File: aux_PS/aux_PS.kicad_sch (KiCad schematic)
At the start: 15 parts, among them J1 P78E03-1000, J2 Conn_02x03_Counter_Clockwise

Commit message: controller_final
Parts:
- AC_DC1, AC_DC2: footprint PSK-S6C-24:PSK-S6C-24 -> PSK-S6C-24:PSKS6C24
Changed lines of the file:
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@@
     (property "Reference" "AC_DC2" (id 0) (at 65.405 55.88 0))
     (property "Value" "PSK-S6C-24" (id 1) (at 65.405 58.42 0))
-    (property "Footprint" "PSK-S6C-24:PSK-S6C-24" (id 2) (at 68.58 71.12 0)
+    (property "Footprint" "PSK-S6C-24:PSKS6C24" (id 2) (at 68.58 71.12 0)
       (effects (font (size 1.27 1.27)) hide)
     )
@@
     (property "Reference" "AC_DC1" (id 0) (at 65.405 38.1 0))
     (property "Value" "PSK-S6C-24" (id 1) (at 65.405 40.64 0))
-    (property "Footprint" "PSK-S6C-24:PSK-S6C-24" (id 2) (at 68.58 53.34 0)
+    (property "Footprint" "PSK-S6C-24:PSKS6C24" (id 2) (at 68.58 53.34 0)
       (effects (font (size 1.27 1.27)) hide)
     )
@@
   (symbol_instances
     (path "/ab1d88f5-8232-454e-a102-ba9788c47905"
-      (reference "AC_DC1") (unit 1) (value "PSK-S6C-24") (footprint "PSK-S6C-24:PSK-S6C-24")
+      (reference "AC_DC1") (unit 1) (value "PSK-S6C-24") (footprint "PSK-S6C-24:PSKS6C24")
     )
     (path "/924609b2-ed56-4d39-928a-34e8ebf74acc"
-      (reference "AC_DC2") (unit 1) (value "PSK-S6C-24") (footprint "PSK-S6C-24:PSK-S6C-24")
+      (reference "AC_DC2") (unit 1) (value "PSK-S6C-24") (footprint "PSK-S6C-24:PSKS6C24")
     )
     (path "/c187c878-09da-4d9b-898f-142200e6ed75"

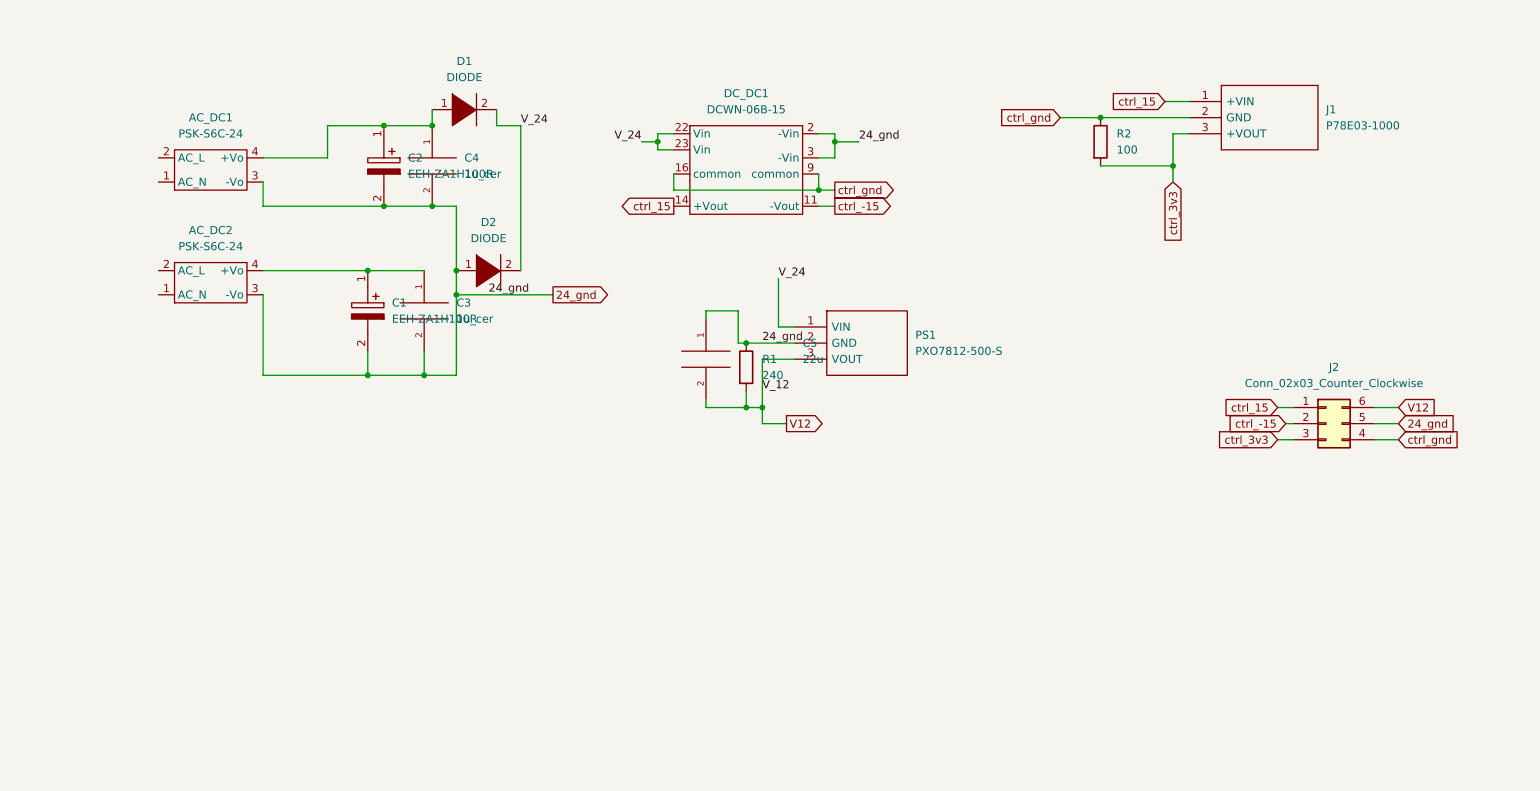
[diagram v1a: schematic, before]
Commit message: header design
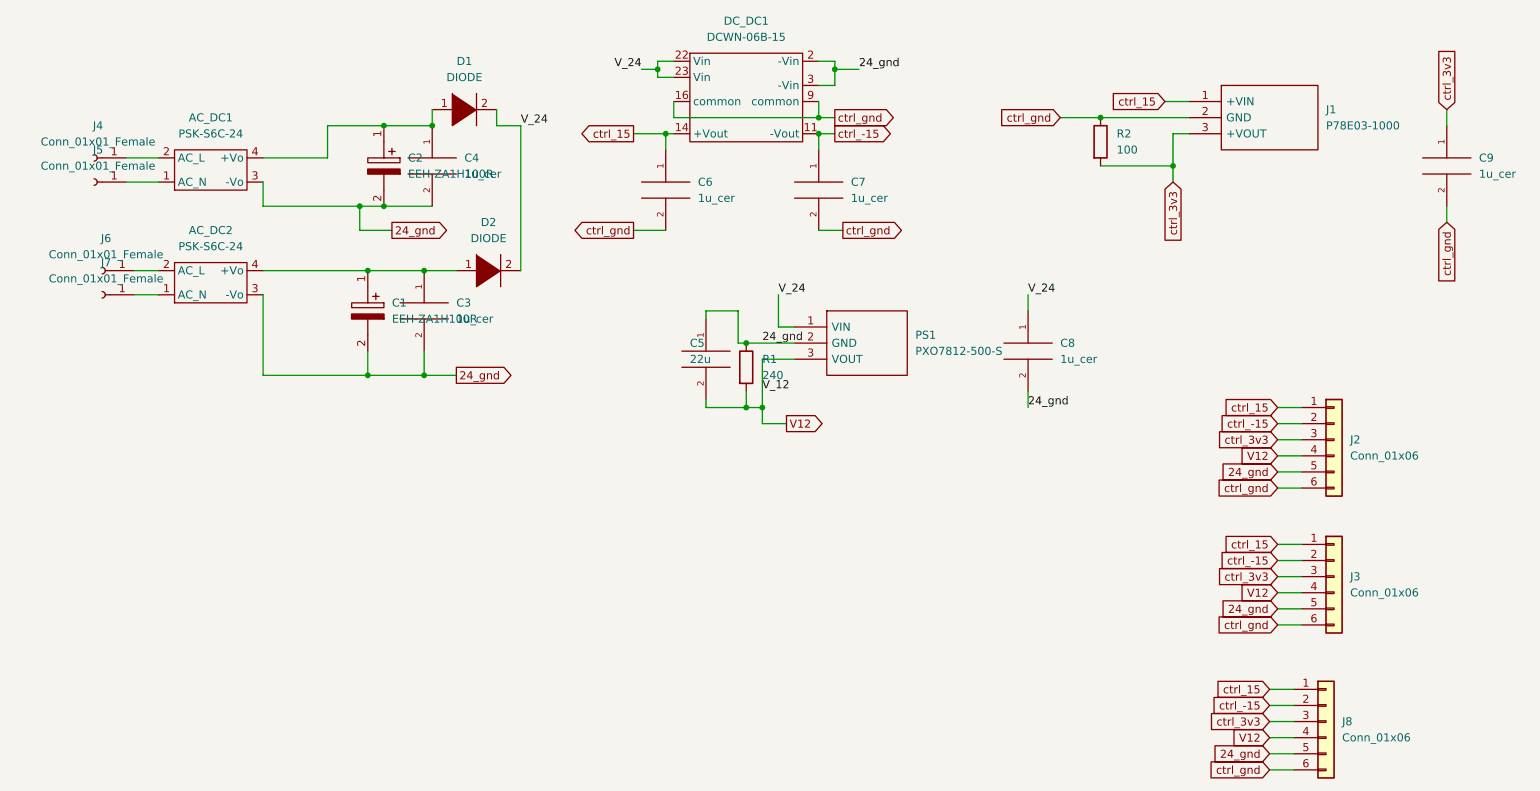
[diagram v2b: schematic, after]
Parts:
- removed J2: Conn_02x03_Counter_Clockwise, Connector_PinSocket_2.54mm:PinSocket_2x03_P2.54mm_Vertical, symbol Connector_Generic:Conn_02x03_Counter_Clockwise
- added C6, C7, C8, C9: 1u_cer, Capacitor_SMD:C_1206_3216Metric_Pad1.33x1.80mm_HandSolder, symbol pspice:CAP
- added J2, J3, J8: Conn_01x06, Connector_PinSocket_2.54mm:PinSocket_1x06_P2.54mm_Vertical, symbol Connector_Generic:Conn_01x06
- added J4, J5, J6, J7: Conn_01x01_Female, Connector:Banana_Jack_1Pin, symbol Connector:Conn_01x01_Female
- C1, C2: footprint EEHZA1H100R -> electro_cap:EEHZA1H100R
- DC_DC1: footprint DCWN-06B:DCWN-06B -> DCWN-06B:DCWN06B15
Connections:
- net 24_gnd: now also C8.2, J2.5 (Pin_5), J3.5 (Pin_5), J8.5 (Pin_5); no longer D2.1 (K)
- net V12: now also J2.4 (Pin_4), J3.4 (Pin_4), J8.4 (Pin_4)
- net V_24: now also C8.1
- net ctrl_-15: now also C7.1, J2.2 (Pin_2), J3.2 (Pin_2), J8.2 (Pin_2)
- net ctrl_15: now also C6.1, J2.1 (Pin_1), J3.1 (Pin_1), J8.1 (Pin_1)
- net ctrl_3v3: now also C9.1, J2.3 (Pin_3), J3.3 (Pin_3), J8.3 (Pin_3)
- net ctrl_gnd: now also C6.2, C7.2, C9.2, J2.6 (Pin_6), J3.6 (Pin_6), J8.6 (Pin_6)
- net at AC_DC2.4 (+Vo), C1.1, C3.1: now also D2.1 (K)
- net at AC_DC2.1 (AC_N): now also J7.1 (Pin_1)
- net at AC_DC2.2 (AC_L): now also J6.1 (Pin_1)
- net at AC_DC1.1 (AC_N): now also J5.1 (Pin_1)
- net at AC_DC1.2 (AC_L): now also J4.1 (Pin_1)
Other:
- moved on the sheet: DC_DC1

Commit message: review changes
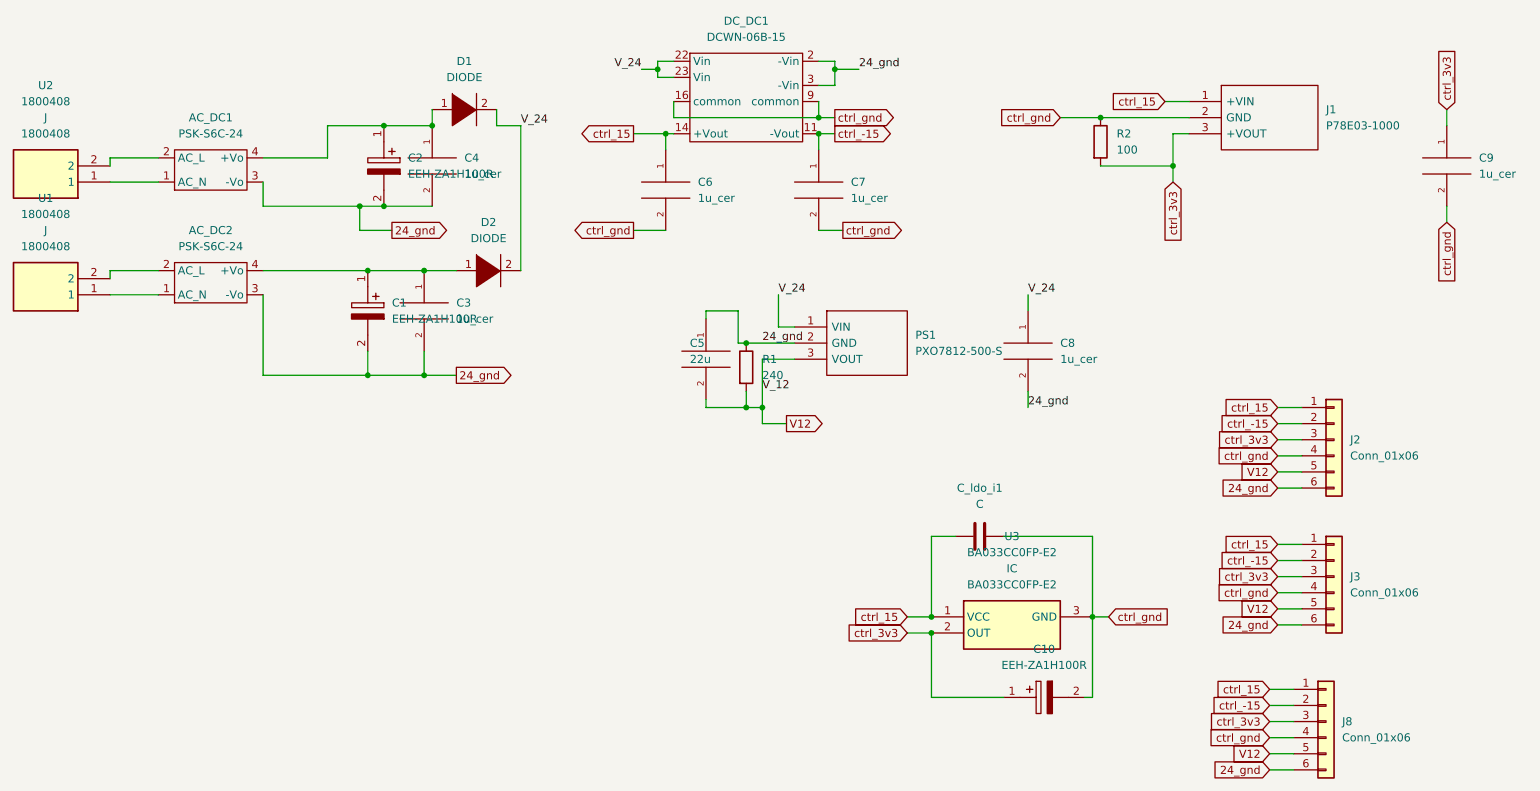
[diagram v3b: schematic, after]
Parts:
- removed J4, J5, J6, J7: Conn_01x01_Female, Connector:Banana_Jack_1Pin, symbol Connector:Conn_01x01_Female
- added C10: EEH-ZA1H100R, electro_cap:EEHZA1H100R, symbol electro_cap:EEH-ZA1H100R
- added C_ldo_i1: C, Capacitor_SMD:C_1206_3216Metric_Pad1.33x1.80mm_HandSolder, symbol Device:C
- added U1, U2: 1800408, power_connector:1800408, symbol connector_power:1800408
- added U3: BA033CC0FP-E2, 3v3_ldo:ROHM_TO-252-3, symbol 3v3_ldo:BA033CC0FP-E2
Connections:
- net 24_gnd: now also J2.6 (Pin_6), J3.6 (Pin_6), J8.6 (Pin_6); no longer J2.5 (Pin_5), J3.5 (Pin_5), J8.5 (Pin_5)
- net V12: now also J2.5 (Pin_5), J3.5 (Pin_5), J8.5 (Pin_5); no longer J2.4 (Pin_4), J3.4 (Pin_4), J8.4 (Pin_4)
- net ctrl_15: now also C_ldo_i1.2, U3.1 (VCC)
- net ctrl_3v3: now also C10.1, U3.2 (OUT)
- net ctrl_gnd: now also J2.4 (Pin_4), J3.4 (Pin_4), J8.4 (Pin_4), C10.2, C_ldo_i1.1, U3.3 (GND); no longer J2.6 (Pin_6), J3.6 (Pin_6), J8.6 (Pin_6)
- net at AC_DC2.1 (AC_N): now also U1.1
- net at AC_DC2.2 (AC_L): now also U1.2
- net at AC_DC1.1 (AC_N): now also U2.1
- net at AC_DC1.2 (AC_L): now also U2.2
